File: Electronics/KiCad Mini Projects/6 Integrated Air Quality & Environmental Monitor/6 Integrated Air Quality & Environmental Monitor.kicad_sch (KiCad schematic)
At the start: 21 parts, among them J1 Power, J10 MQ4, J11 MQ5, J12 MQ6, J13 MQ7, J14 MQ8, J15 MQ9, J16 MQ135, J17 MQ139, J18 KY028, J19 DHT11, J2 PWM, J20 DHT11, J21 BMP180, J3 Analog, J4 PWM, J5 Analog, J6 Communication, J7 Screw_Terminal_01x02, J8 MQ2, J9 MQ3

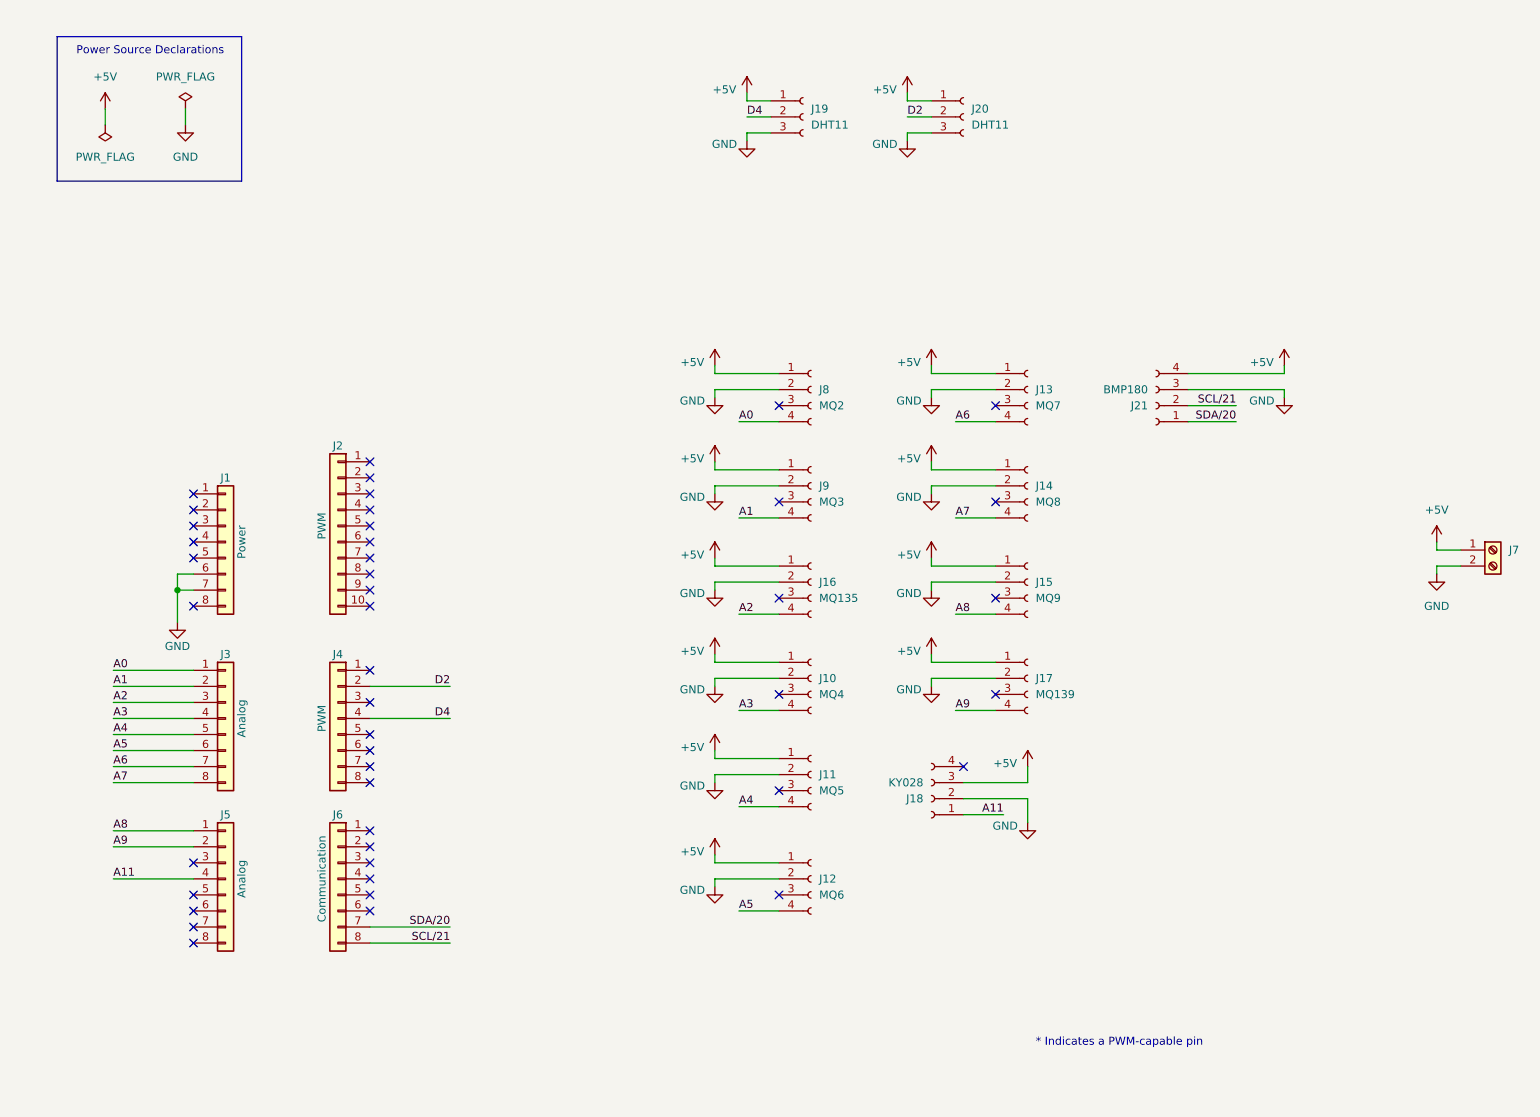
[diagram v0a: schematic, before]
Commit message: KiCad Mini Projects files
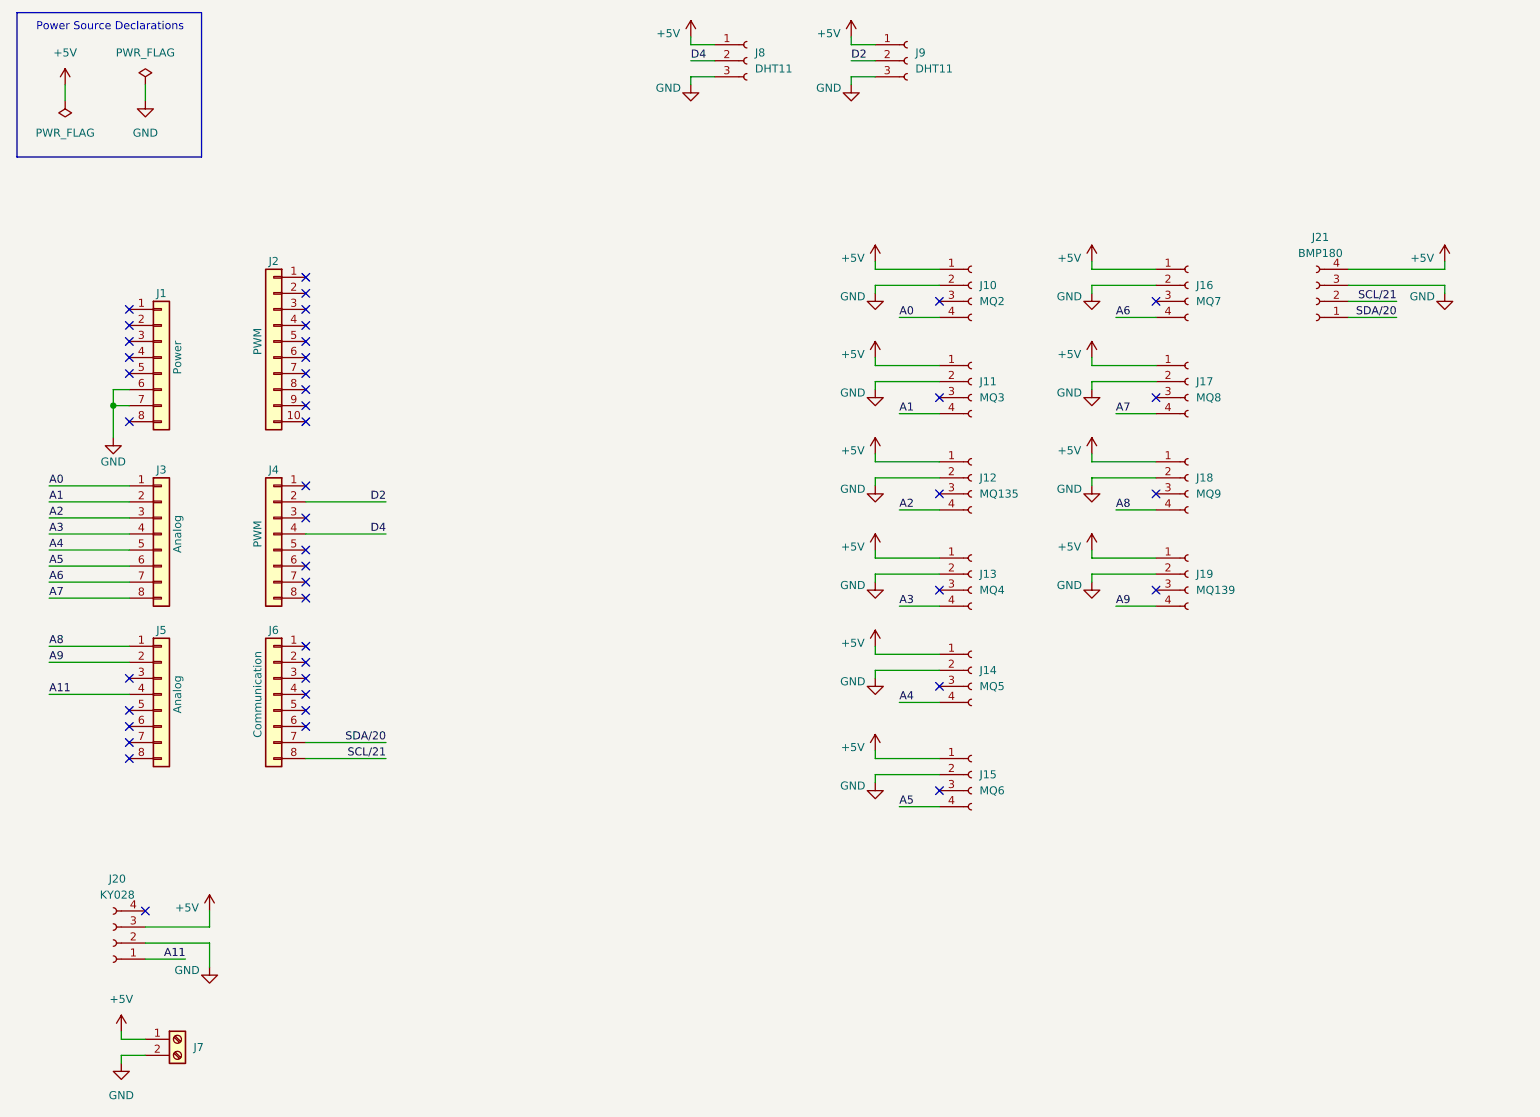
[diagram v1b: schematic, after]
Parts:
- removed J19, J20: DHT11, Connector_PinSocket_2.54mm:PinSocket_1x03_P2.54mm_Vertical, symbol Connector:Conn_01x03_Socket
- removed J8: MQ2, Connector_PinSocket_2.54mm:PinSocket_1x04_P2.54mm_Vertical, symbol Connector:Conn_01x04_Socket
- removed J9: MQ3, Connector_PinSocket_2.54mm:PinSocket_1x04_P2.54mm_Vertical, symbol Connector:Conn_01x04_Socket
- added J19: MQ139, Connector_PinHeader_2.54mm:PinHeader_1x04_P2.54mm_Vertical, symbol Connector:Conn_01x04_Socket
- added J20: KY028, Connector_PinSocket_2.54mm:PinSocket_1x04_P2.54mm_Vertical, symbol Connector:Conn_01x04_Socket
- added J8, J9: DHT11, Connector_PinSocket_2.54mm:PinSocket_1x03_P2.54mm_Vertical, symbol Connector:Conn_01x03_Socket
- J10: value MQ4 -> MQ2; footprint Connector_PinSocket_2.54mm:PinSocket_1x04_P2.54mm_Vertical -> My Library:MQ_Module_Vertical
- J11: value MQ5 -> MQ3; footprint Connector_PinSocket_2.54mm:PinSocket_1x04_P2.54mm_Vertical -> My Library:MQ_Module_Vertical
- J12: value MQ6 -> MQ135; footprint Connector_PinSocket_2.54mm:PinSocket_1x04_P2.54mm_Vertical -> My Library:MQ_Module_Vertical
- J13: value MQ7 -> MQ4
- J14: value MQ8 -> MQ5
- J15: value MQ9 -> MQ6; footprint Connector_PinSocket_2.54mm:PinSocket_1x04_P2.54mm_Vertical -> My Library:MQ_Module_Vertical
- J16: value MQ135 -> MQ7; footprint Connector_PinSocket_2.54mm:PinSocket_1x04_P2.54mm_Vertical -> My Library:MQ_Module_Vertical
- J17: value MQ139 -> MQ8; footprint Connector_PinSocket_2.54mm:PinSocket_1x04_P2.54mm_Vertical -> My Library:MQ_Module_Vertical
- J18: value KY028 -> MQ9
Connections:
- net +5V: now also J18.1 (Pin_1), J19.1 (Pin_1), J20.3 (Pin_3), J8.1 (Pin_1), J9.1 (Pin_1); no longer J18.3 (Pin_3)
- net A0: now also J10.4 (Pin_4)
- net A1: now also J11.4 (Pin_4)
- net A11: now also J20.1 (Pin_1); no longer J18.1 (Pin_1)
- net A2: now also J12.4 (Pin_4); no longer J16.4 (Pin_4)
- net A3: now also J13.4 (Pin_4); no longer J10.4 (Pin_4)
- net A4: now also J14.4 (Pin_4); no longer J11.4 (Pin_4)
- net A5: now also J15.4 (Pin_4); no longer J12.4 (Pin_4)
- net A6: now also J16.4 (Pin_4); no longer J13.4 (Pin_4)
- net A7: now also J17.4 (Pin_4); no longer J14.4 (Pin_4)
- net A8: now also J18.4 (Pin_4); no longer J15.4 (Pin_4)
- net A9: now also J19.4 (Pin_4); no longer J17.4 (Pin_4)
- net D2: now also J9.2 (Pin_2)
- net D4: now also J8.2 (Pin_2)
- net GND: now also J19.2 (Pin_2), J20.2 (Pin_2), J8.3 (Pin_3), J9.3 (Pin_3)
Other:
- note removed: "* Indicates a PWM-capable pin"
- title: (none) -> Integrated Air Quality & Environmental Monitor
